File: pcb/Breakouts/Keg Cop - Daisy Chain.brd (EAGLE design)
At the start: 45 x 51 mm, 9 parts, among them X2 RJ45-8X

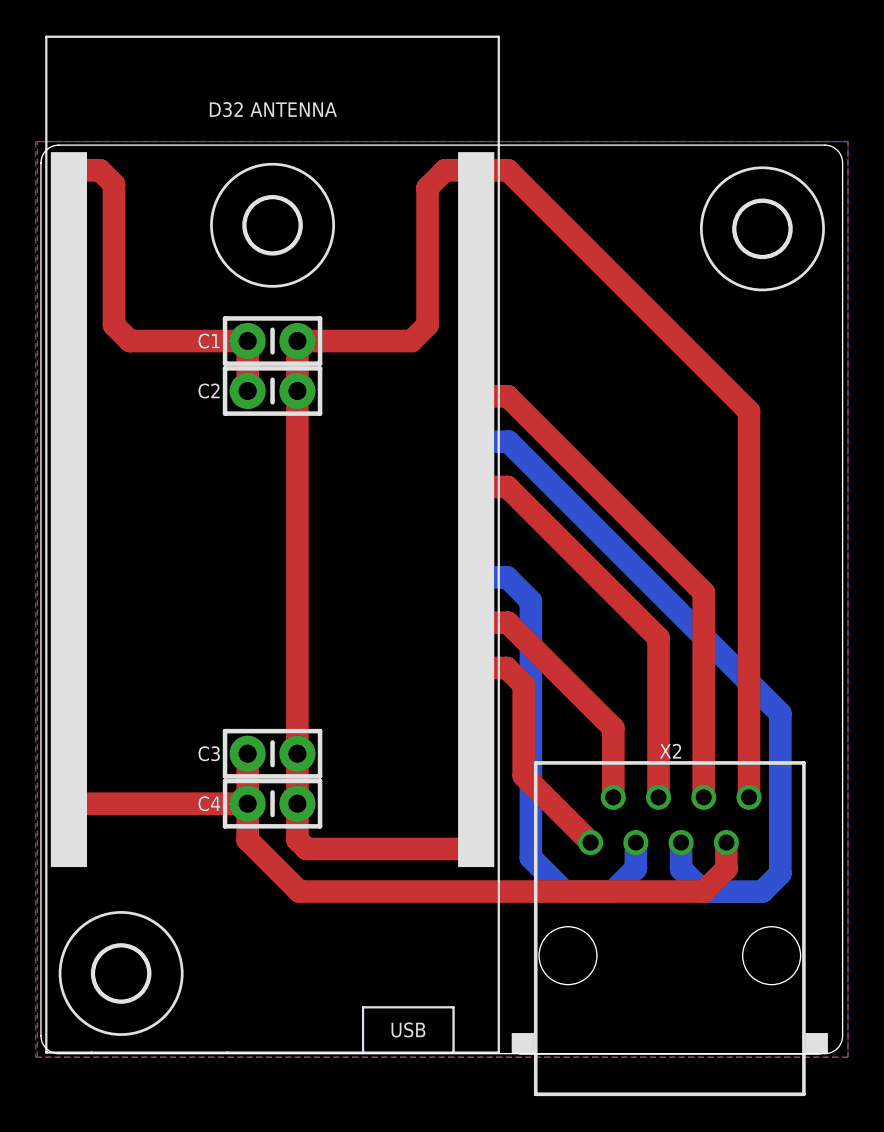
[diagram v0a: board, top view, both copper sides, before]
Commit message: Rename files
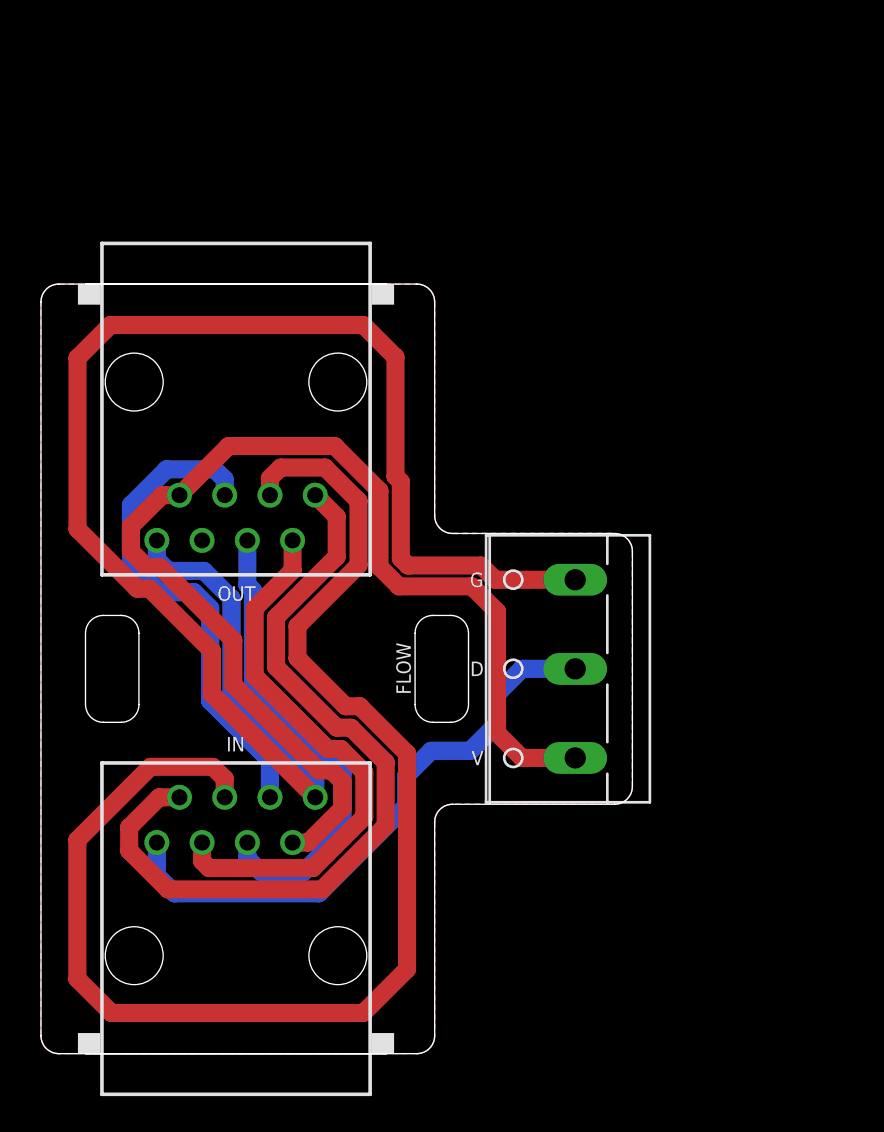
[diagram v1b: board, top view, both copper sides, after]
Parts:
- removed C1, C3: 0.1μF, Donnie:CAP_PTH-2.54
- removed C2, C4: 1.0μF, Donnie:CAP_PTH-2.54
- removed D32: Lolin D32, Donnie:D32_NO_BATT
- removed U$1, U$2, U$3: (no value), holes:3,0
- removed X2: RJ45-8X, con-tycoelectronics:RJ45-NO-SHIELD
- added FLOW: (no value), con-wago-500:W237-103
- added IN, OUT: RJ45-8X, con-tycoelectronics:RJ45-NO-SHIELD
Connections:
- removed net KEG1: D32.IO4, X2.1
- removed net KEG2: D32.IO16, X2.2
- removed net KEG3: D32.IO17, X2.3
- removed net KEG4: D32.IO18, X2.4
- removed net KEG5: D32.IO19, X2.5
- removed net KEG6: D32.IO21, X2.6
- removed net VCC: C1.1, C2.1, D32.VCC
- new net DATA: FLOW.2, IN.1
- new net N$1: IN.2, OUT.1
- new net N$2: IN.3, OUT.2
- new net N$3: IN.4, OUT.3
- new net N$5: IN.5, OUT.4
- new net N$7: IN.6, OUT.5
- net 5V: now also FLOW.1, IN.7, OUT.7; no longer C3.1, C4.1, D32.VBUS, X2.7
- net GND: now also FLOW.3, IN.8, OUT.8; no longer C1.2, C2.2, C3.2, C4.2, D32.GND, D32.GND2, X2.8
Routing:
- net N$3: track 0.00 -> 77.1 mm
- net N$1: track 0.00 -> 45.1 mm
- net KEG5: track 40.4 -> 0.00 mm
- net DATA: track 0.00 -> 33.0 mm
- net N$2: track 0.00 -> 30.9 mm
- net KEG6: track 28.8 -> 0.00 mm
- net N$7: track 0.00 -> 28.0 mm
- net KEG3: track 26.7 -> 0.00 mm
- net N$5: track 0.00 -> 26.1 mm
- net KEG4: track 22.7 -> 0.00 mm
- net VCC: track 21.4 -> 0.00 mm
- net 5V: track 44.9 -> 65.7 mm
- net KEG2: track 14.0 -> 0.00 mm
- net KEG1: track 13.5 -> 0.00 mm
- net GND: track 99.3 -> 90.9 mm
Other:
- board size 45 x 51 mm -> 33.2 x 43.2 mm
- board text added: "D"
- board text added: "G"
- board text added: "V"
- board text removed: "1 - KEG1 2 - KEG2 3 - KEG3 4 - KEG4"
- board text removed: "5 - KEG5 6 - KEG6 7 - KEG7 8 - KEG8"
